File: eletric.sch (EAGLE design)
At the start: 13 parts, among them U1 ATTINY85-20PU

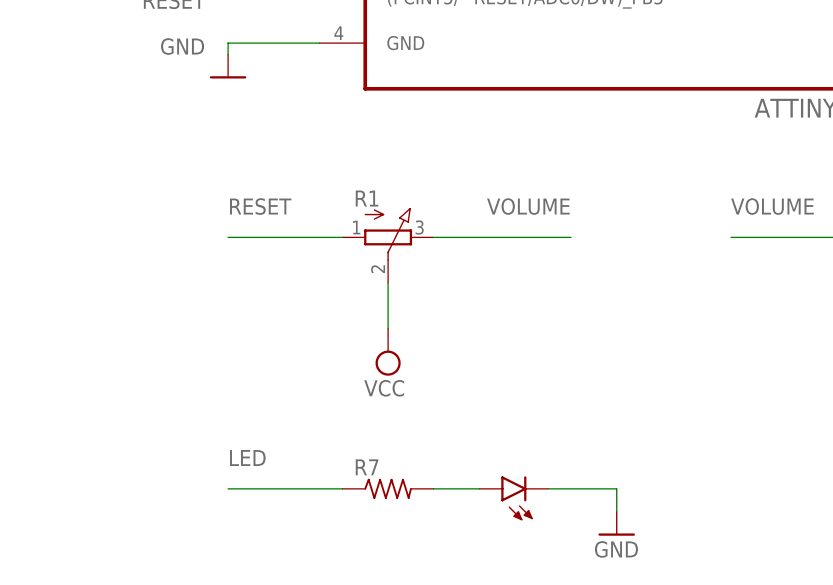
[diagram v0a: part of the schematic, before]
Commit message: pcb improve layout
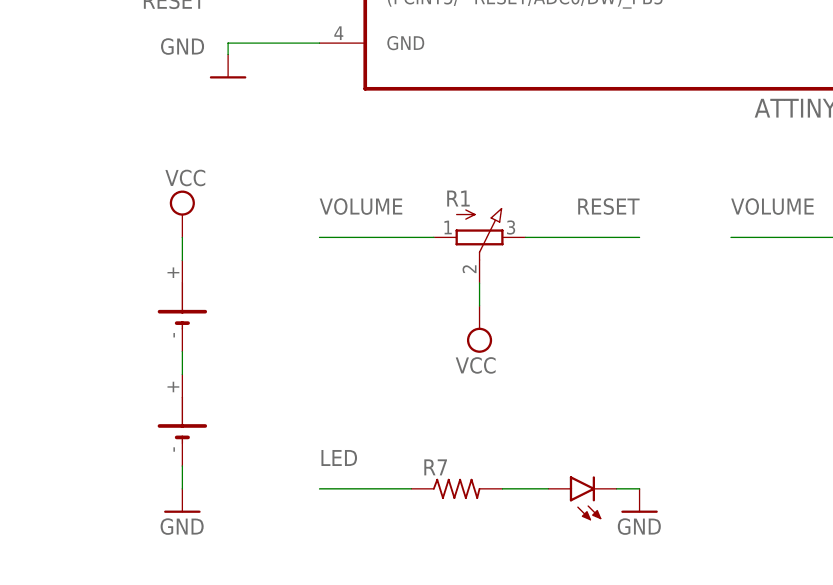
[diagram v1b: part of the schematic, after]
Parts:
- removed LED2: (no value), led:LED5MM
- added G1, G2: CR-AA, battery:CR-AA
- added LED1: (no value), led:LED3MM
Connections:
- new net N$1: G1.-, G2.+
- net GND: now also G2.-, LED1.C; no longer LED2.C
- net N$5: now also LED1.A; no longer LED2.A
- net RESET: now also R1.E; no longer R1.A
- net VCC: now also G1.+
- net VOLUME: now also R1.A; no longer R1.E
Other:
- moved on the sheet: R1, R7
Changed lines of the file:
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@@
 </classes>
 <parts>
-<part name="LED2" library="led" library_urn="urn:adsk.eagle:library:259" deviceset="LED" device="5MM" package3d_urn="urn:adsk.eagle:package:15799/2"/>
 <part name="LS1" library="CMT-8530S-SMT" deviceset="CMT-8530S-SMT" device=""/>
 <part name="LS2" library="CMT-8530S-SMT" deviceset="CMT-8530S-SMT" device=""/>
@@
 <part name="R6" library="rcl" library_urn="urn:adsk.eagle:library:334" deviceset="R-US_" device="R0805" package3d_urn="urn:adsk.eagle:package:23553/2"/>
 <part name="R7" library="rcl" library_urn="urn:adsk.eagle:library:334" deviceset="R-US_" device="R0805" package3d_urn="urn:adsk.eagle:package:23553/2"/>
+<part name="G1" library="battery" library_urn="urn:adsk.eagle:library:109" deviceset="CR-AA" device="" package3d_urn="urn:adsk.eagle:package:4582/2"/>
+<part name="G2" library="battery" library_urn="urn:adsk.eagle:library:109" deviceset="CR-AA" device="" package3d_urn="urn:adsk.eagle:package:4582/2"/>
+<part name="GND3" library="supply1" library_urn="urn:adsk.eagle:library:371" deviceset="GND" device=""/>
+<part name="SUPPLY3" library="supply2" library_urn="urn:adsk.eagle:library:372" deviceset="VCC" device=""/>
+<part name="LED1" library="led" library_urn="urn:adsk.eagle:library:259" deviceset="LED" device="3MM" package3d_urn="urn:adsk.eagle:package:15797/1"/>
 </parts>
 <sheets>
@@
 </plain>
 <instances>
-<instance part="LED2" gate="G$1" x="-15.24" y="-15.24" smashed="yes" rot="R90">
-<attribute name="VALUE" x="-10.668" y="-9.525" size="1.778" layer="96" rot="R180"/>
-</instance>
 <instance part="LS1" gate="G$1" x="66.04" y="-17.78" smashed="yes" rot="R90"/>
 <instance part="LS2" gate="G$1" x="66.04" y="12.7" smashed="yes" rot="R90"/>
@@
 <attribute name="VALUE" x="-48.26" y="33.02" size="1.778" layer="96" align="bottom-right"/>
 </instance>
-<instance part="R1" gate="G$1" x="-27.94" y="12.7" smashed="yes" rot="R270">
-<attribute name="NAME" x="-31.75" y="16.129" size="1.778" layer="95"/>
-<attribute name="VALUE" x="-31.75" y="16.51" size="1.778" layer="96"/>
-</instance>
-<instance part="SUPPLY2" gate="G$1" x="-27.94" y="0" smashed="yes" rot="R180">
-<attribute name="VALUE" x="-26.035" y="-3.175" size="1.778" layer="96" rot="R180"/>
-</instance>
-<instance part="GND2" gate="1" x="-2.54" y="-20.32" smashed="yes">
-<attribute name="VALUE" x="-5.08" y="-22.86" size="1.778" layer="96"/>
+<instance part="R1" gate="G$1" x="-17.78" y="12.7" smashed="yes" rot="R270">
+<attribute name="NAME" x="-21.59" y="16.129" size="1.778" layer="95"/>
+<attribute name="VALUE" x="-21.59" y="16.51" size="1.778" layer="96"/>
+</instance>
+<instance part="SUPPLY2" gate="G$1" x="-17.78" y="2.54" smashed="yes" rot="R180">
+<attribute name="VALUE" x="-15.875" y="-0.635" size="1.778" layer="96" rot="R180"/>
+</instance>
+<instance part="GND2" gate="1" x="0" y="-17.78" smashed="yes">
+<attribute name="VALUE" x="-2.54" y="-20.32" size="1.778" layer="96"/>
 </instance>
 <instance part="R2" gate="G$1" x="40.64" y="12.7" smashed="yes">
@@
 <attribute name="VALUE" x="36.83" y="-13.462" size="1.778" layer="96"/>
 </instance>
-<instance part="R7" gate="G$1" x="-27.94" y="-15.24" smashed="yes">
-<attribute name="NAME" x="-31.75" y="-13.7414" size="1.778" layer="95"/>
-<attribute name="VALUE" x="-31.75" y="-18.542" size="1.778" layer="96"/>
+<instance part="R7" gate="G$1" x="-20.32" y="-15.24" smashed="yes">
+<attribute name="NAME" x="-24.13" y="-13.7414" size="1.778" layer="95"/>
+<attribute name="VALUE" x="-24.13" y="-18.542" size="1.778" layer="96"/>
+</instance>
+<instance part="G1" gate="1" x="-50.8" y="5.08" smashed="yes" rot="R90"/>
+<instance part="G2" gate="1" x="-50.8" y="-7.62" smashed="yes" rot="R90"/>
+<instance part="GND3" gate="1" x="-50.8" y="-17.78" smashed="yes">
+<attribute name="VALUE" x="-53.34" y="-20.32" size="1.778" layer="96"/>
+</instance>
+<instance part="SUPPLY3" gate="G$1" x="-50.8" y="15.24" smashed="yes">
+<attribute name="VALUE" x="-52.705" y="18.415" size="1.778" layer="96"/>
+</instance>
+<instance part="LED1" gate="G$1" x="-7.62" y="-15.24" smashed="yes" rot="R90">
+<attribute name="VALUE" x="-3.048" y="-9.525" size="1.778" layer="96" rot="R180"/>
 </instance>
 </instances>
@@
 <nets>
 <net name="VOLUME" class="0">
-<segment>
-<pinref part="R1" gate="G$1" pin="E"/>
-<wire x1="-22.86" y1="12.7" x2="-7.62" y2="12.7" width="0.1524" layer="91"/>
-<label x="-7.62" y="15.24" size="1.778" layer="95" align="bottom-right"/>
-</segment>
 <segment>
 <wire x1="35.56" y1="12.7" x2="22.86" y2="12.7" width="0.1524" layer="91"/>
@@
 <junction x="22.86" y="-10.16"/>
 </segment>
+<segment>
+<pinref part="R1" gate="G$1" pin="A"/>
+<wire x1="-22.86" y1="12.7" x2="-35.56" y2="12.7" width="0.1524" layer="91"/>
+<label x="-35.56" y="15.24" size="1.778" layer="95"/>
+</segment>
 </net>
 <net name="VCC" class="0">
@@
 <pinref part="R1" gate="G$1" pin="S"/>
 <pinref part="SUPPLY2" gate="G$1" pin="VCC"/>
-<wire x1="-27.94" y1="7.62" x2="-27.94" y2="2.54" width="0.1524" layer="91"/>
+<wire x1="-17.78" y1="7.62" x2="-17.78" y2="5.08" width="0.1524" layer="91"/>
+</segment>
+<segment>
+<pinref part="SUPPLY3" gate="G$1" pin="VCC"/>
+<pinref part="G1" gate="1" pin="+"/>
+<wire x1="-50.8" y1="12.7" x2="-50.8" y2="10.16" width="0.1524" layer="91"/>
 </segment>
 </net>
@@
 </segment>
 <segment>
-<pinref part="LED2" gate="G$1" pin="C"/>
 <pinref part="GND2" gate="1" pin="GND"/>
-<wire x1="-10.16" y1="-15.24" x2="-2.54" y2="-15.24" width="0.1524" layer="91"/>
-<wire x1="-2.54" y1="-15.24" x2="-2.54" y2="-17.78" width="0.1524" layer="91"/>
+<wire x1="-2.54" y1="-15.24" x2="0" y2="-15.24" width="0.1524" layer="91"/>
+<pinref part="LED1" gate="G$1" pin="C"/>
+</segment>
+<segment>
+<pinref part="G2" gate="1" pin="-"/>
+<pinref part="GND3" gate="1" pin="GND"/>
+<wire x1="-50.8" y1="-12.7" x2="-50.8" y2="-15.24" width="0.1524" layer="91"/>
 </segment>
 </net>
 <net name="LED" class="0">
 <segment>
-<wire x1="-33.02" y1="-15.24" x2="-45.72" y2="-15.24" width="0.1524" layer="91"/>
-<label x="-45.72" y="-12.7" size="1.778" layer="95"/>
+<wire x1="-25.4" y1="-15.24" x2="-35.56" y2="-15.24" width="0.1524" layer="91"/>
+<label x="-35.56" y="-12.7" size="1.778" layer="95"/>
 <pinref part="R7" gate="G$1" pin="1"/>
 </segment>
@@
 <net name="RESET" class="0">
 <segment>
-<pinref part="R1" gate="G$1" pin="A"/>
-<wire x1="-33.02" y1="12.7" x2="-45.72" y2="12.7" width="0.1524" layer="91"/>
-<label x="-45.72" y="15.24" size="1.778" layer="95"/>
-</segment>
-<segment>
 <pinref part="U1" gate="A" pin="(PCINT5/~RESET/ADC0/DW)_PB5"/>
 <wire x1="-35.56" y1="39.37" x2="-45.72" y2="39.37" width="0.1524" layer="91"/>
 <label x="-48.26" y="38.1" size="1.778" layer="95" align="bottom-right"/>
 </segment>
+<segment>
+<pinref part="R1" gate="G$1" pin="E"/>
+<wire x1="-12.7" y1="12.7" x2="0" y2="12.7" width="0.1524" layer="91"/>
+<label x="0" y="15.24" size="1.778" layer="95" align="bottom-right"/>
+</segment>
 </net>
 <net name="N$5" class="0">
 <segment>
-<pinref part="LED2" gate="G$1" pin="A"/>
-<wire x1="-22.86" y1="-15.24" x2="-17.78" y2="-15.24" width="0.1524" layer="91"/>
 <pinref part="R7" gate="G$1" pin="2"/>
+<wire x1="-10.16" y1="-15.24" x2="-15.24" y2="-15.24" width="0.1524" layer="91"/>
+<pinref part="LED1" gate="G$1" pin="A"/>
 </segment>
 </net>
@@
 </segment>
 </net>
+<net name="N$1" class="0">
+<segment>
+<pinref part="G1" gate="1" pin="-"/>
+<pinref part="G2" gate="1" pin="+"/>
+<wire x1="-50.8" y1="0" x2="-50.8" y2="-2.54" width="0.1524" layer="91"/>
+</segment>
+</net>
